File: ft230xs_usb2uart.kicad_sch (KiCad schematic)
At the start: 19 parts, among them J1 USB_A, J2 Conn_01x02_Socket, U3 FT230XS

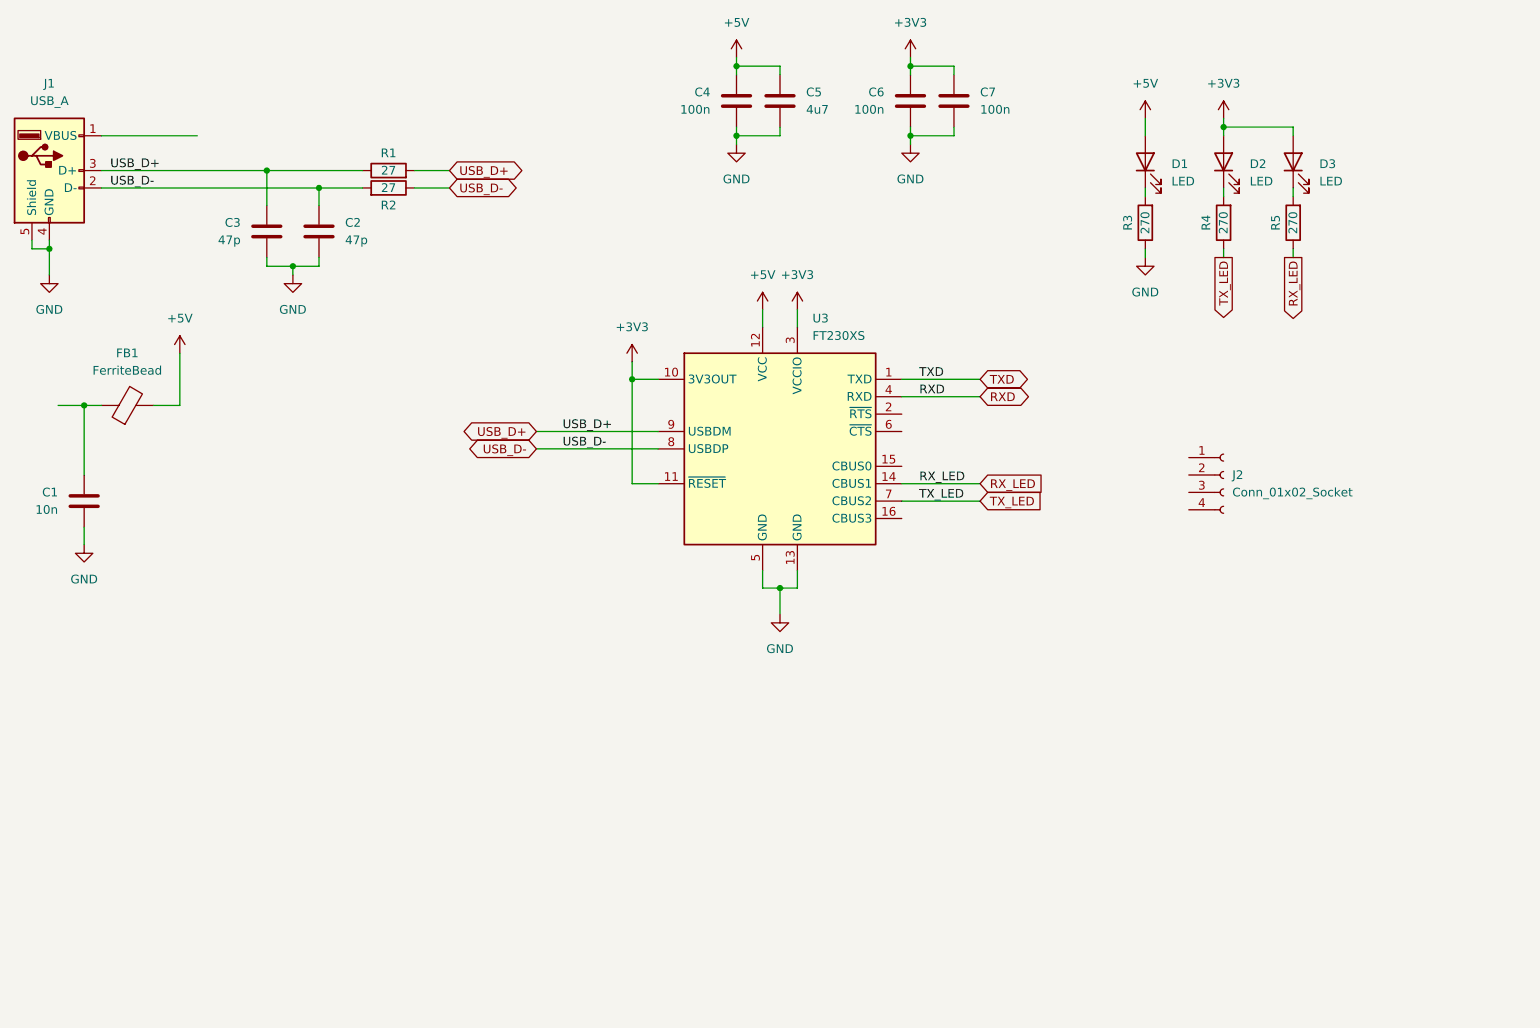
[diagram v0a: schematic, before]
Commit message: asdasd
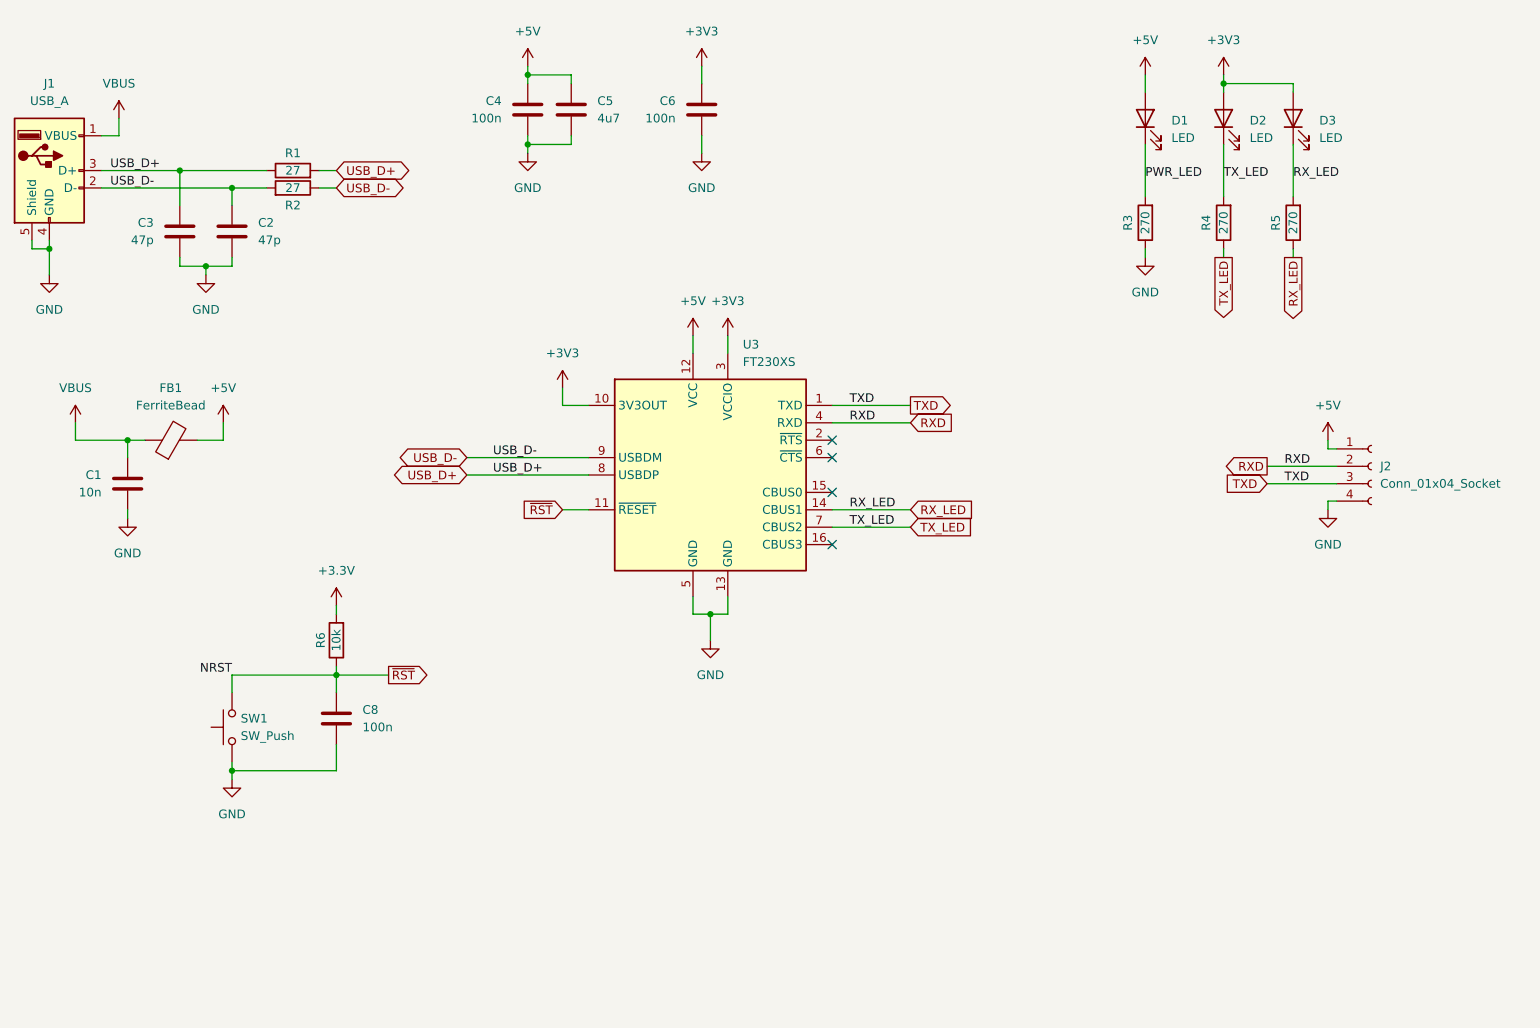
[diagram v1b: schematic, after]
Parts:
- removed C7: 100n, symbol Device:C
- added C8: 100n, Capacitor_SMD:C_0603_1608Metric, symbol Device:C
- added R6: 10k, Resistor_SMD:R_0603_1608Metric_Pad0.98x0.95mm_HandSolder, symbol Device:R
- added SW1: SW_Push, Button_Switch_SMD:SW_Push_SPST_NO_Alps_SKRK, symbol Switch:SW_Push
- C2, C3, C4, C5, C6: footprint (none) -> Capacitor_SMD:C_0603_1608Metric_Pad1.08x0.95mm_HandSolder
- D1, D2, D3: footprint (none) -> LED_SMD:LED_0603_1608Metric_Pad1.05x0.95mm_HandSolder
- J2: value Conn_01x02_Socket -> Conn_01x04_Socket; footprint Connector_PinSocket_2.54mm:PinSocket_1x04_P2.54mm_Vertical -> Connector_JST:JST_XH_S4B-XH-A_1x04_P2.50mm_Horizontal
- R1, R2, R3, R4, R5: footprint (none) -> Resistor_SMD:R_0603_1608Metric_Pad0.98x0.95mm_HandSolder
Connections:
- net +3V3: no longer U3.11 (~{RESET})
- net +5V: now also J2.1 (Pin_1)
- net GND: now also J2.4 (Pin_4), C8.2, SW1.1
- net RXD: now also J2.2 (Pin_2)
- net RX_LED: now also D3.1 (K), R5.2
- net TXD: now also J2.3 (Pin_3)
- net TX_LED: now also D2.1 (K), R4.2
- net USB_D+: now also U3.8 (USBDP); no longer U3.9 (USBDM)
- net USB_D-: now also U3.9 (USBDM); no longer U3.8 (USBDP)
- net VBUS: now reaches C1.1, FB1.1
- net VBUS: now also J1.1 (VBUS)
- net PWR_LED: now reaches D1.1 (K), R3.2
- new net +3.3V: R6.2
- new net ~{RST}: C8.1, R6.1, SW1.2, U3.11 (~{RESET})
- no-connect marks 0 -> 4
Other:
- moved on the sheet: C1, C2, C3, C4, C5, C6, D1, D2, D3, FB1, R1, R2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

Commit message: adasd
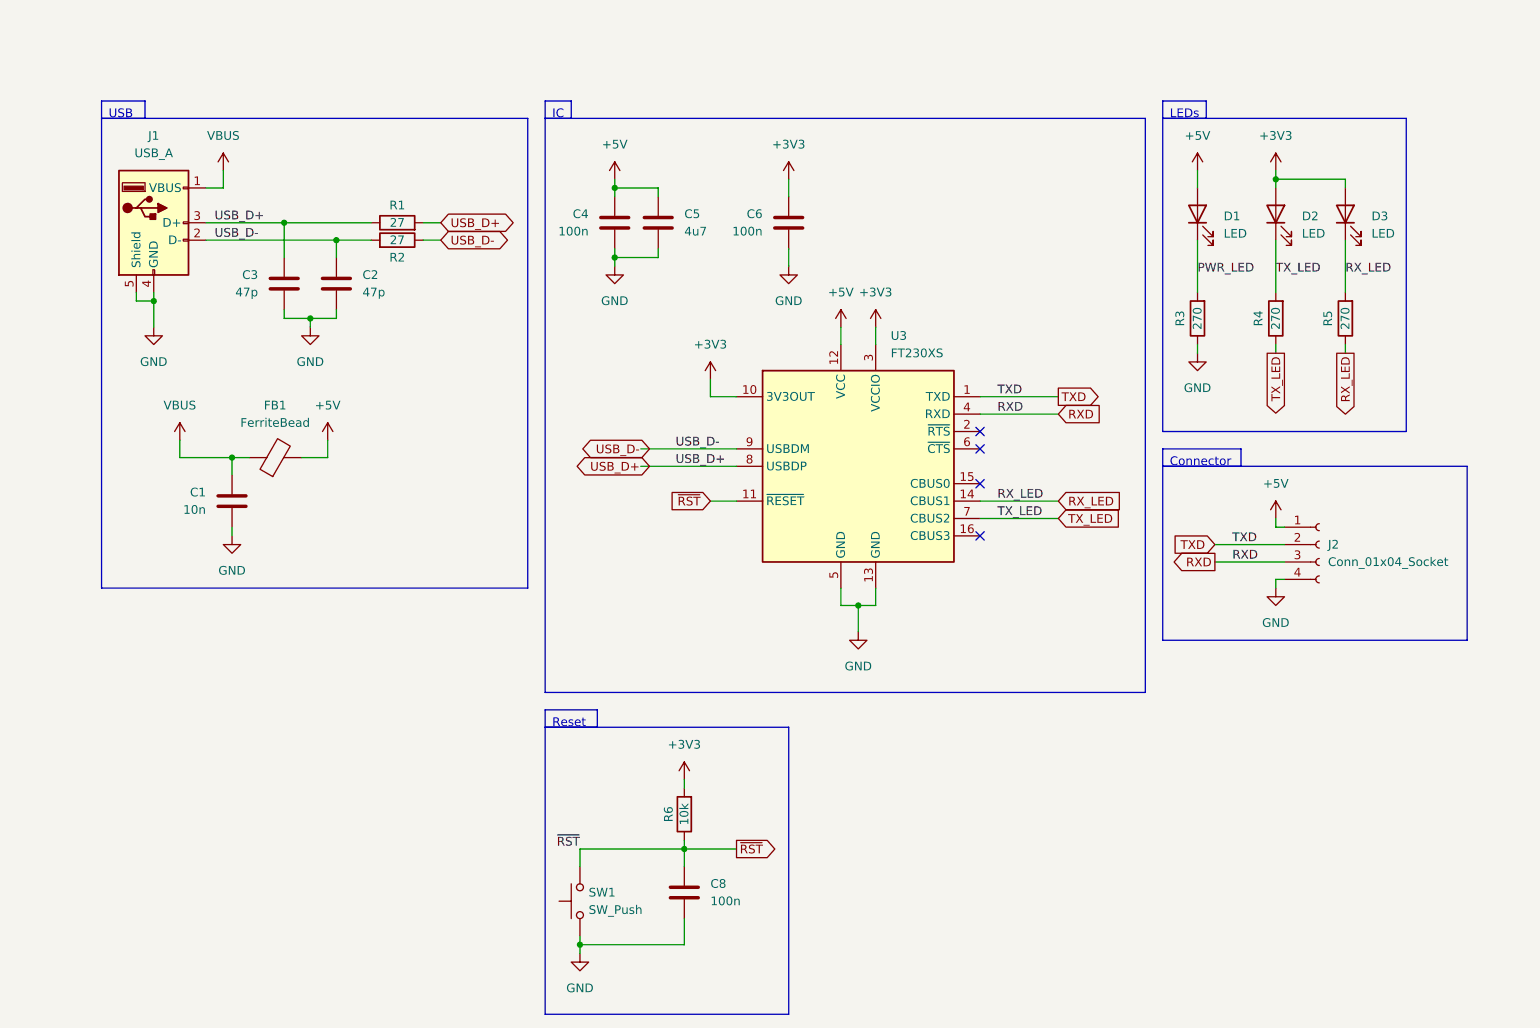
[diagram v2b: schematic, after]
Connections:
- net +3.3V is gone; now on net +3V3: R6.2
- net RXD: now also J2.3 (Pin_3); no longer J2.2 (Pin_2)
- net TXD: now also J2.2 (Pin_2); no longer J2.3 (Pin_3)
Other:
- company: (none) -> KAJDEV
- title: (none) -> USB2UART
- moved on the sheet: C1, C2, C3, C4, C5, C6, C8, D1, D2, D3, FB1, J1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
